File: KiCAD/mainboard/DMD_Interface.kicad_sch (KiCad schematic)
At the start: 13 parts, among them J1 AXT550124, J30 Conn_01x08_Pin

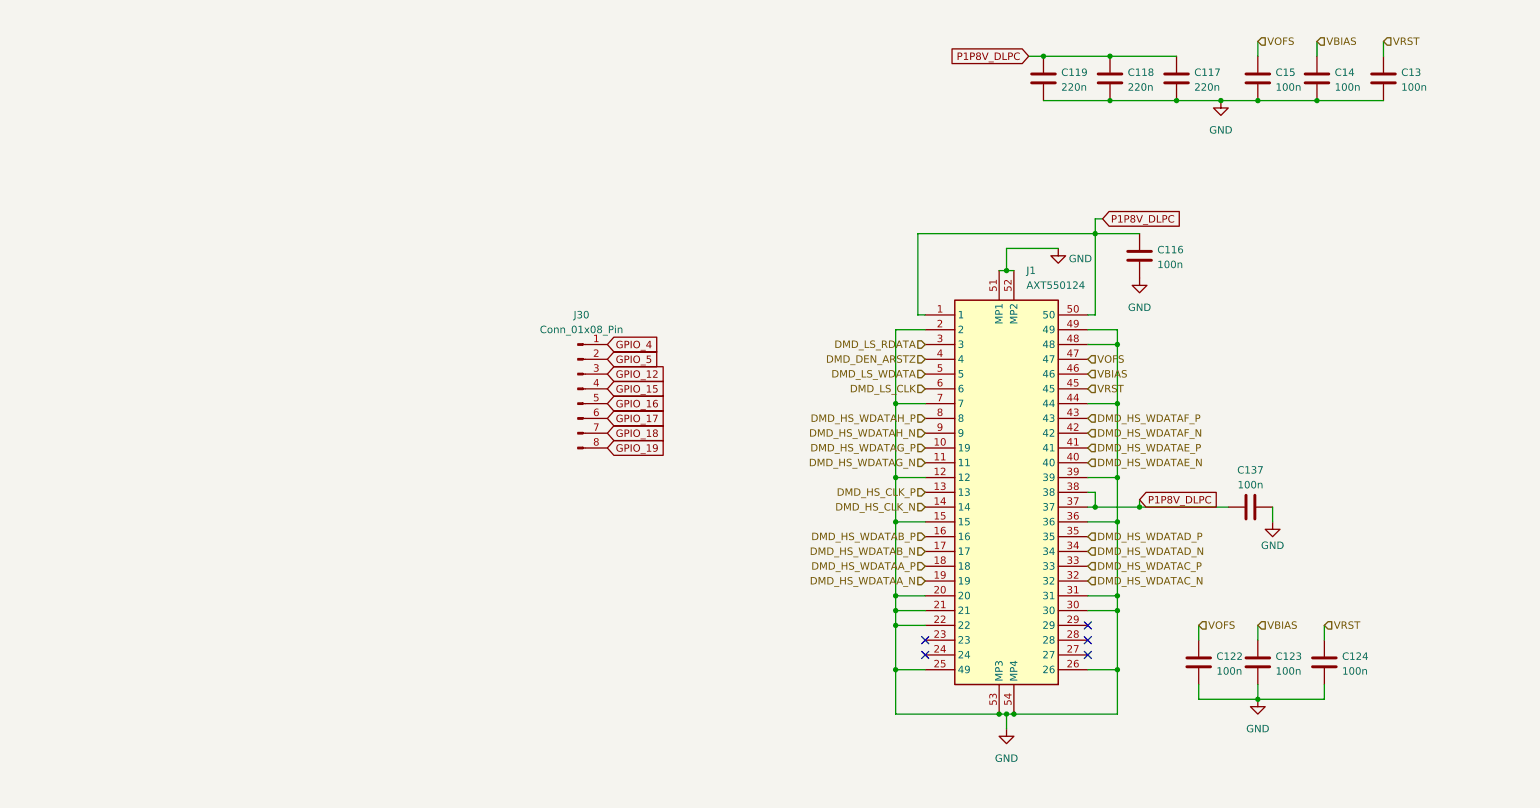
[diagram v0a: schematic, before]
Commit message: dmd interface done!
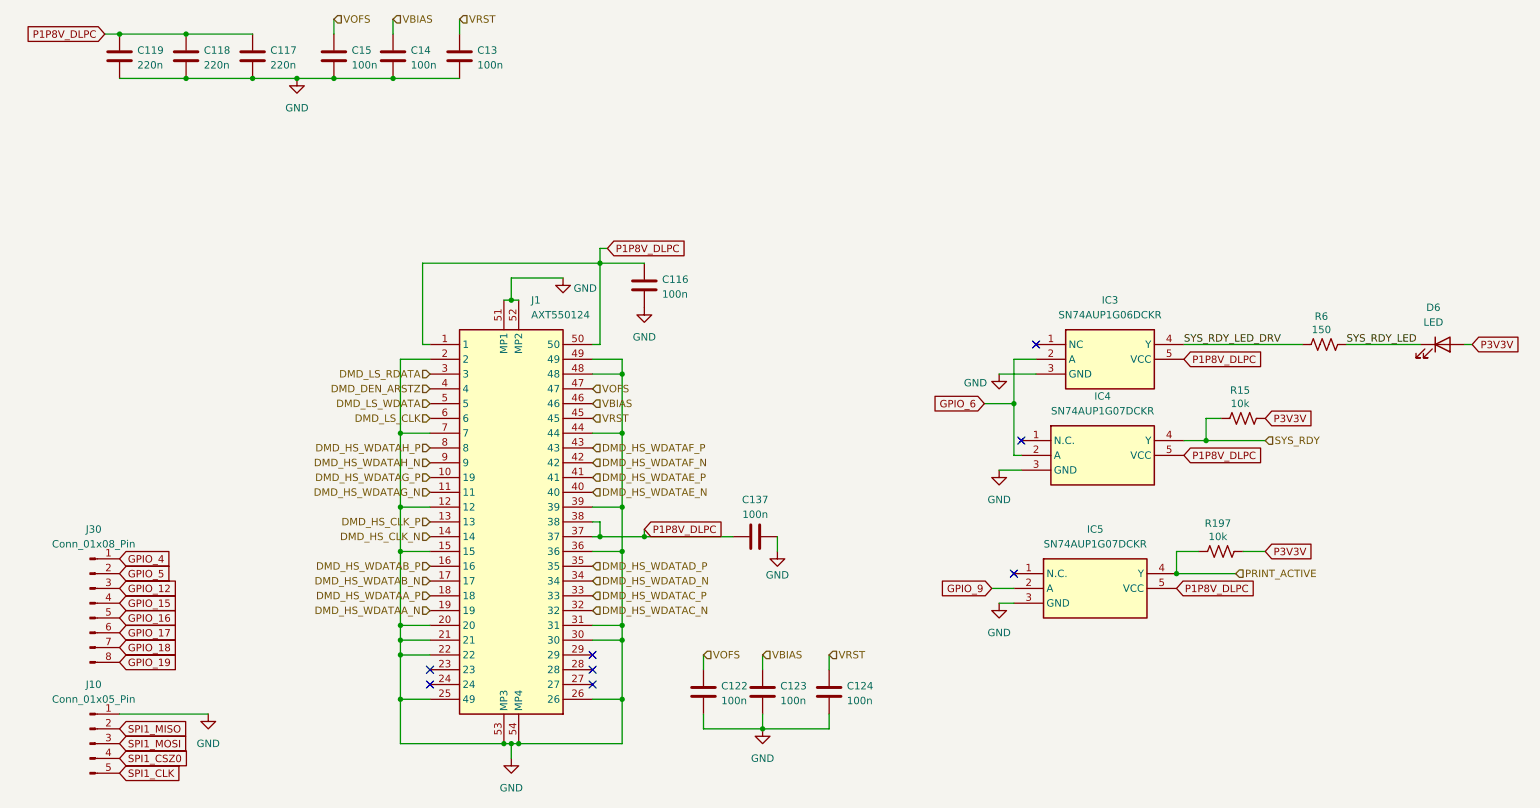
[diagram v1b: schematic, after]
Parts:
- added D6: LED, LED_SMD:LED_1206_3216Metric, symbol Device:LED
- added IC3: SN74AUP1G06DCKR, tp_library:SOT65P210X110-5N, symbol tp_library:SN74AUP1G06DCKR
- added IC4, IC5: SN74AUP1G07DCKR, tp_library:SOT65P210X110-5N, symbol tp_library:SN74AUP1G07DCKR
- added J10: Conn_01x05_Pin, Connector_PinHeader_2.54mm:PinHeader_1x05_P2.54mm_Vertical, symbol Connector:Conn_01x05_Pin
- added R15, R197: 10k, Resistor_SMD:R_0402_1005Metric, symbol Device:R_US
- added R6: 150, Resistor_SMD:R_0402_1005Metric, symbol Device:R_US
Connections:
- net GND: now also IC3.3 (GND), IC4.3 (GND), IC5.3 (GND), J10.1 (Pin_1)
- net P1P8V_DLPC: now also IC3.5 (VCC), IC4.5 (VCC), IC5.5 (VCC)
- new net GPIO_6: IC3.2 (A), IC4.2 (A)
- new net GPIO_9: IC5.2 (A)
- new net P3V3V: D6.2 (A), R15.1, R197.1
- new net PRINT_ACTIVE: IC5.4 (Y), R197.2
- new net SPI1_CLK: J10.5 (Pin_5)
- new net SPI1_CSZ0: J10.4 (Pin_4)
- new net SPI1_MISO: J10.2 (Pin_2)
- new net SPI1_MOSI: J10.3 (Pin_3)
- new net SYS_RDY: IC4.4 (Y), R15.2
- new net SYS_RDY_LED: D6.1 (K), R6.1
- new net SYS_RDY_LED_DRV: IC3.4 (Y), R6.2
- no-connect marks 5 -> 8
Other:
- moved on the sheet: C116, C117, C118, C119, C122, C123, C124, C13, C137, C14, C15, J1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
